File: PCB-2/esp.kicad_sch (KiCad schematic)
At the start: 7 parts, among them J1 FFC, J11 SMA (WiFi), U8 NINA-W101

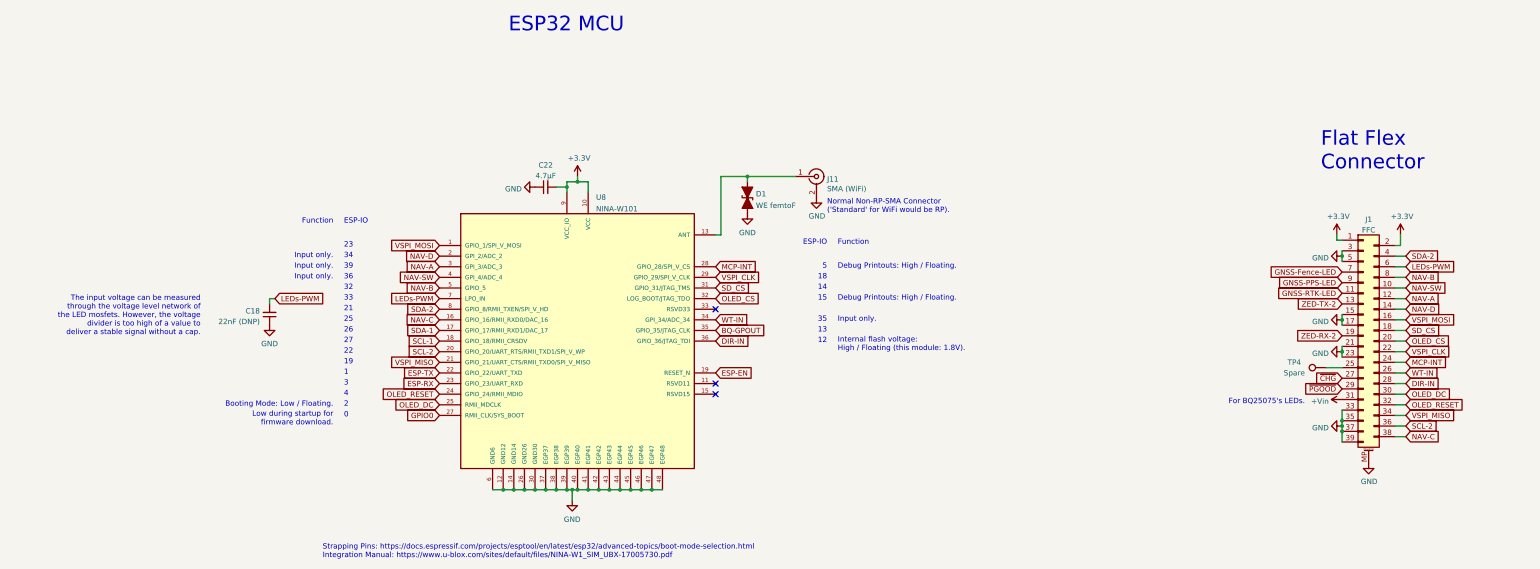
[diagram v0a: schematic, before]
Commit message: added photos to docu
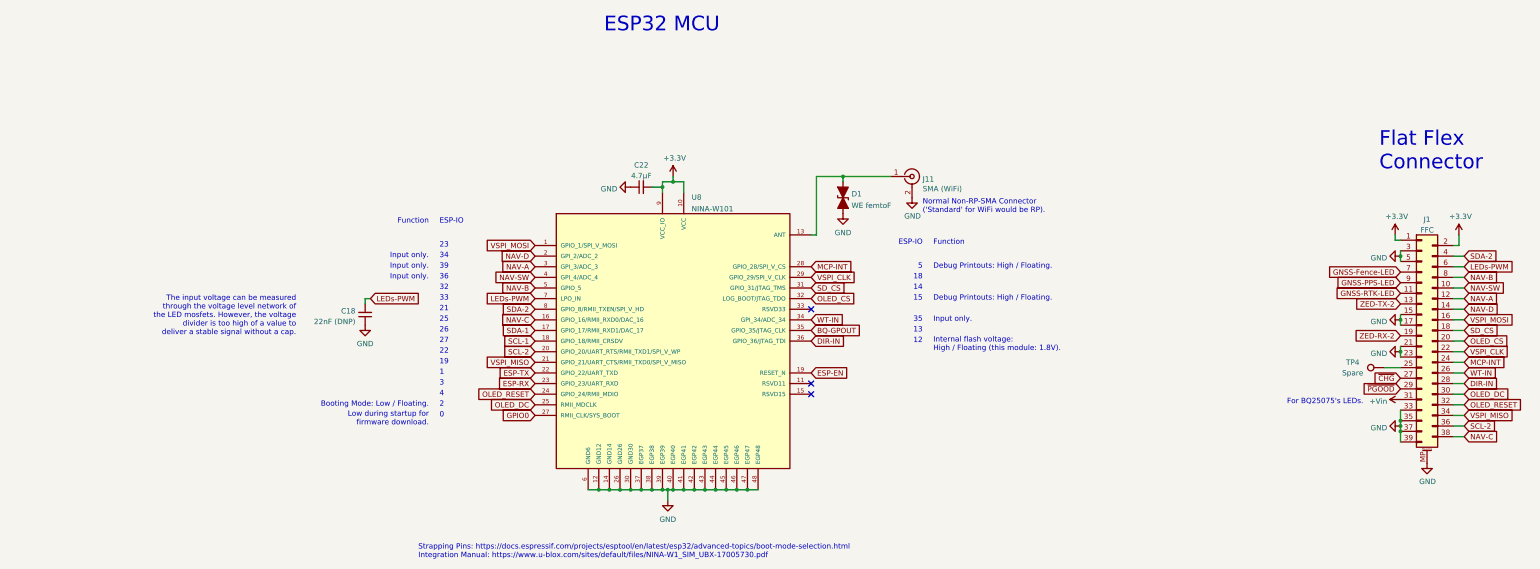
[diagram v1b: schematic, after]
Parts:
- C18: footprint (none) -> Franz-Lib:C_0402_1005Metric_NoSilk_DNP
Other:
- moved on the sheet: C18, C22, D1, J1, J11, TP4, U8
